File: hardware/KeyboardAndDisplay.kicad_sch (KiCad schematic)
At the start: 34 parts, among them SW301 Q/1/STOP, SW302 W/2/CH0, SW303 E/3/CH1, SW304 R/4/CH2, SW305 T/5/CH3, SW306 Y/6/_, SW307 U/7/-, SW308 I/8/+, SW309 O/9/=, SW310 P/0, SW311 A/!/`, SW312 S/"/CH4, SW313 D/$/CH5, SW314 F/%/CH6, SW315 G/^/CH7, SW316 H/&/{, SW317 J/*/}, SW318 K/(/[, SW319 L/)/], SW320 BKSP/DEL, SW321 SHIFT, SW322 Z/\/|, SW323 X/;/:, SW324 C/'/@, SW325 V/#/~, SW326 B/,/<, SW327 N/./>, SW328 M///?, SW329 SYM, SW330 SPC/ENT, U301 MCP23S17_SP, U302 NHD-0420DZ-FL-YBW

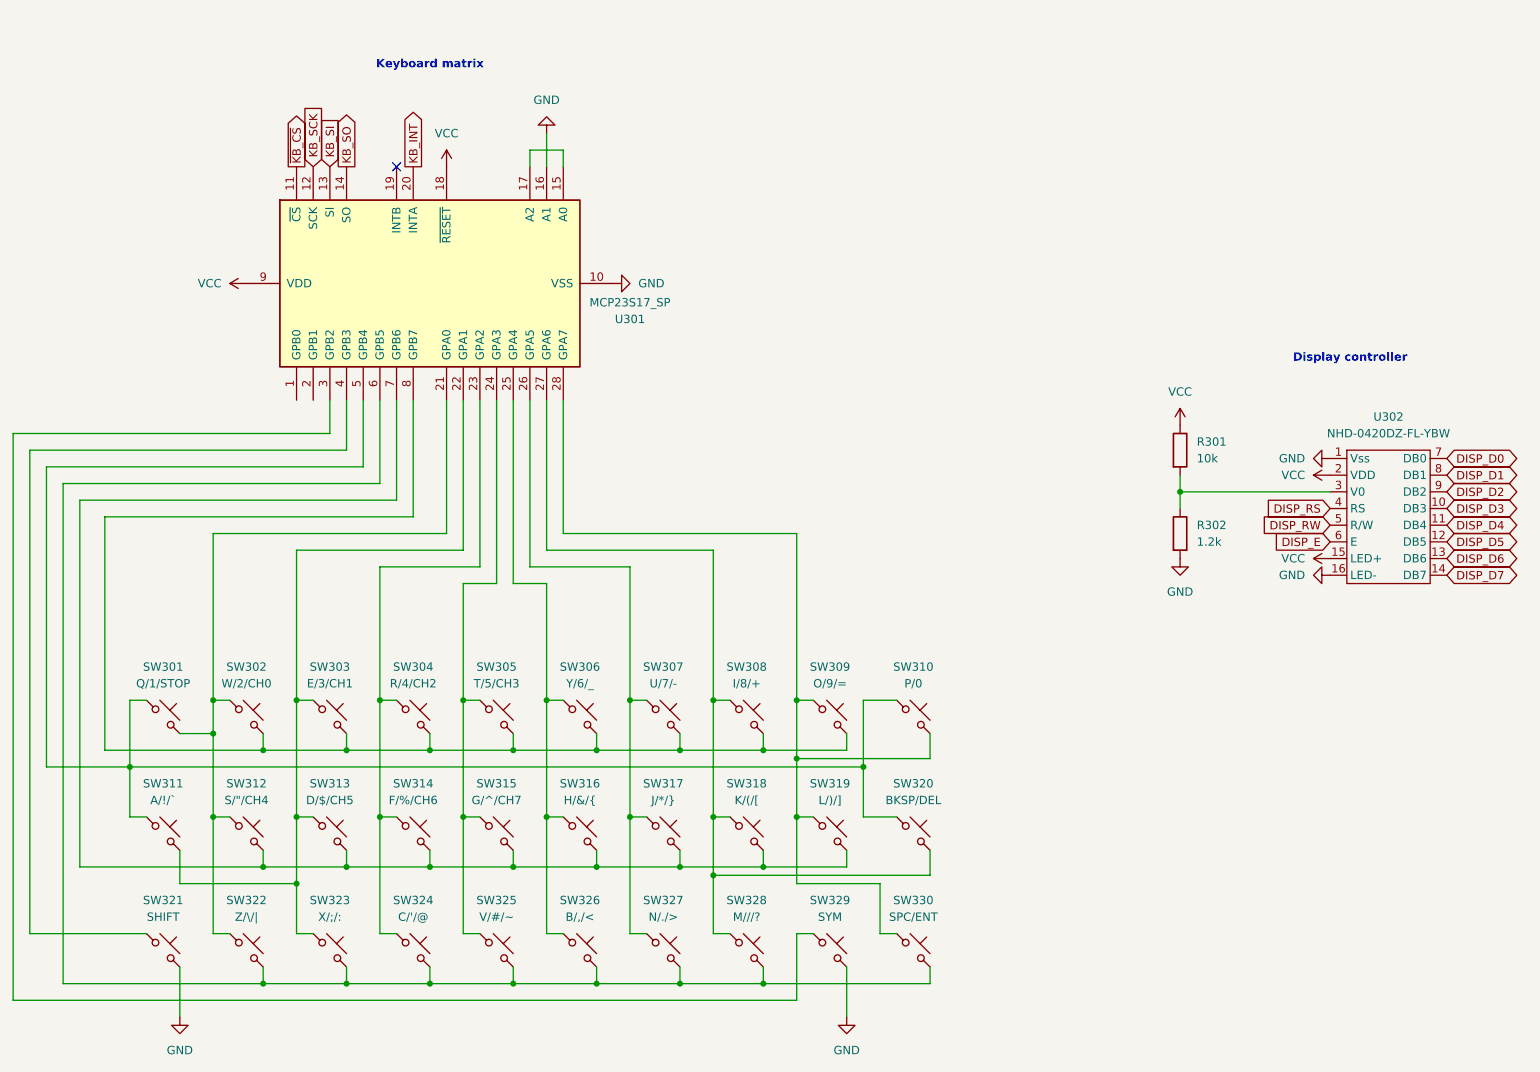
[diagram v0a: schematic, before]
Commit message: Add final planned components
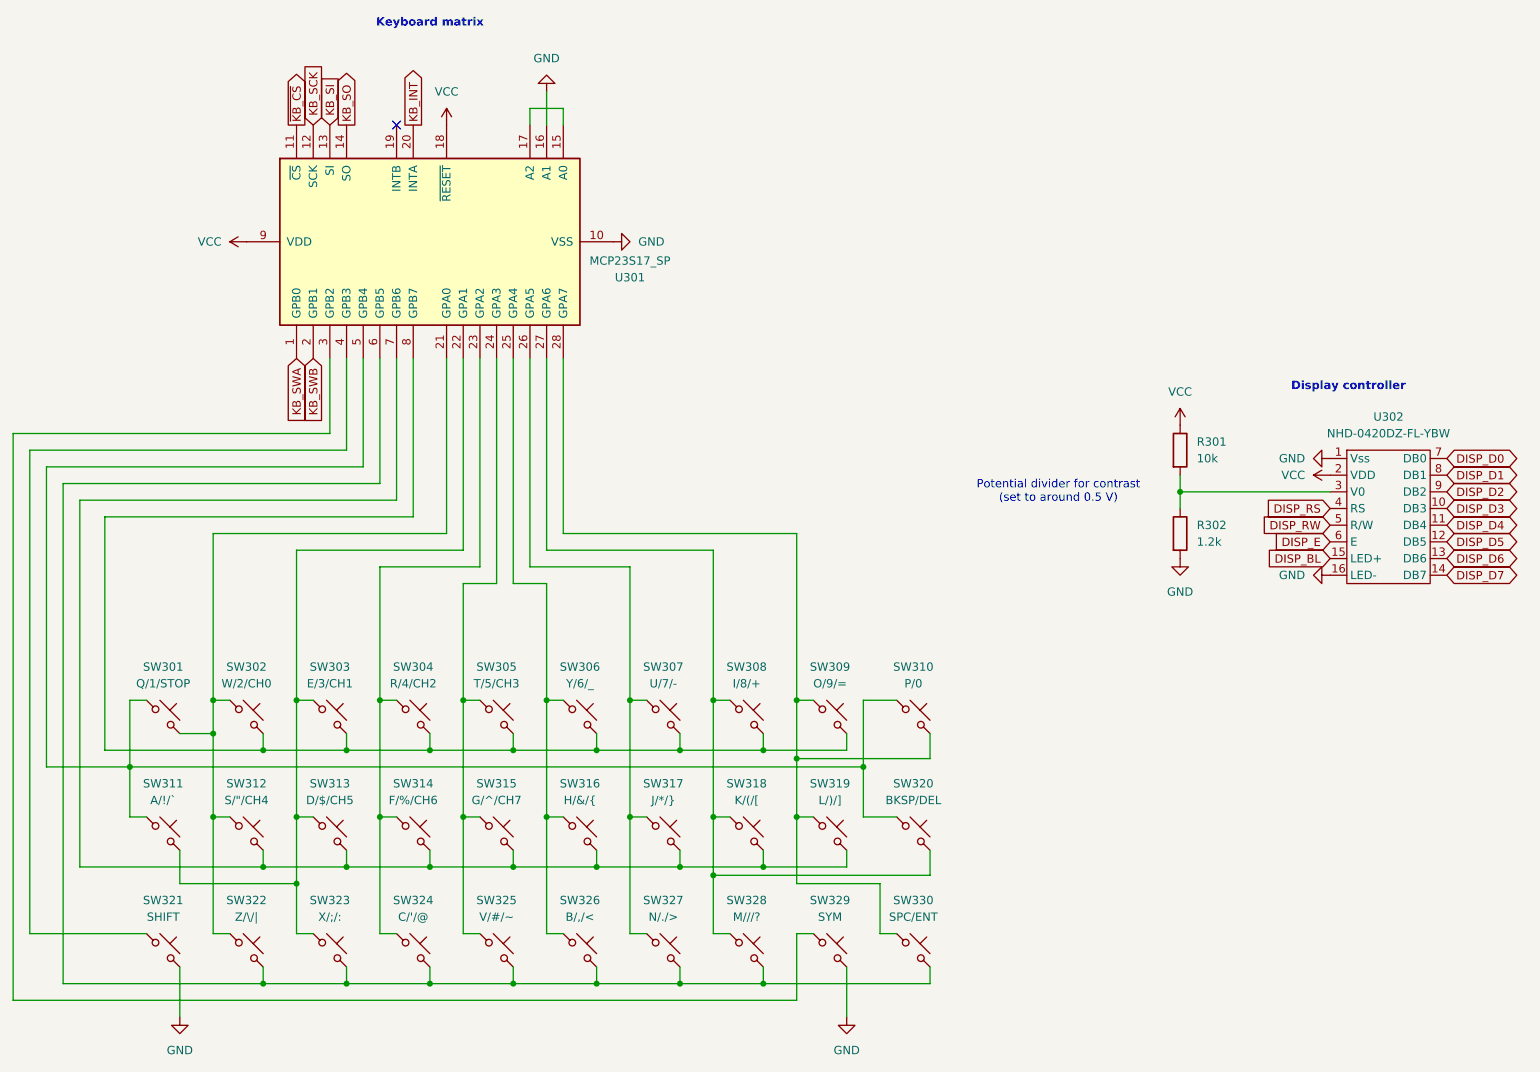
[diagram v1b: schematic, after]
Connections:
- net VCC: no longer U302.15 (LED+)
- net KB_SWA: now reaches U301.1 (GPB0)
- net KB_SWB: now reaches U301.2 (GPB1)
- new net DISP_BL: U302.15 (LED+)
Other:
- note added: "Potential divider for contrast (set to around 0.5 V)"
- moved on the sheet: U301
